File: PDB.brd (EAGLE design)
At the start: 126.8 x 162.5 mm, 49 parts, among them J1 B06B-HCMKK, J2 B06B-HCMKK, J3 SS-6488-NF-A431, J4 SS-6488-NF-A431, J5 B06B-HCMKK, J6 B03B-HCMKS, J7 B03B-HCMKS, J8 SS-6488-NF-A431

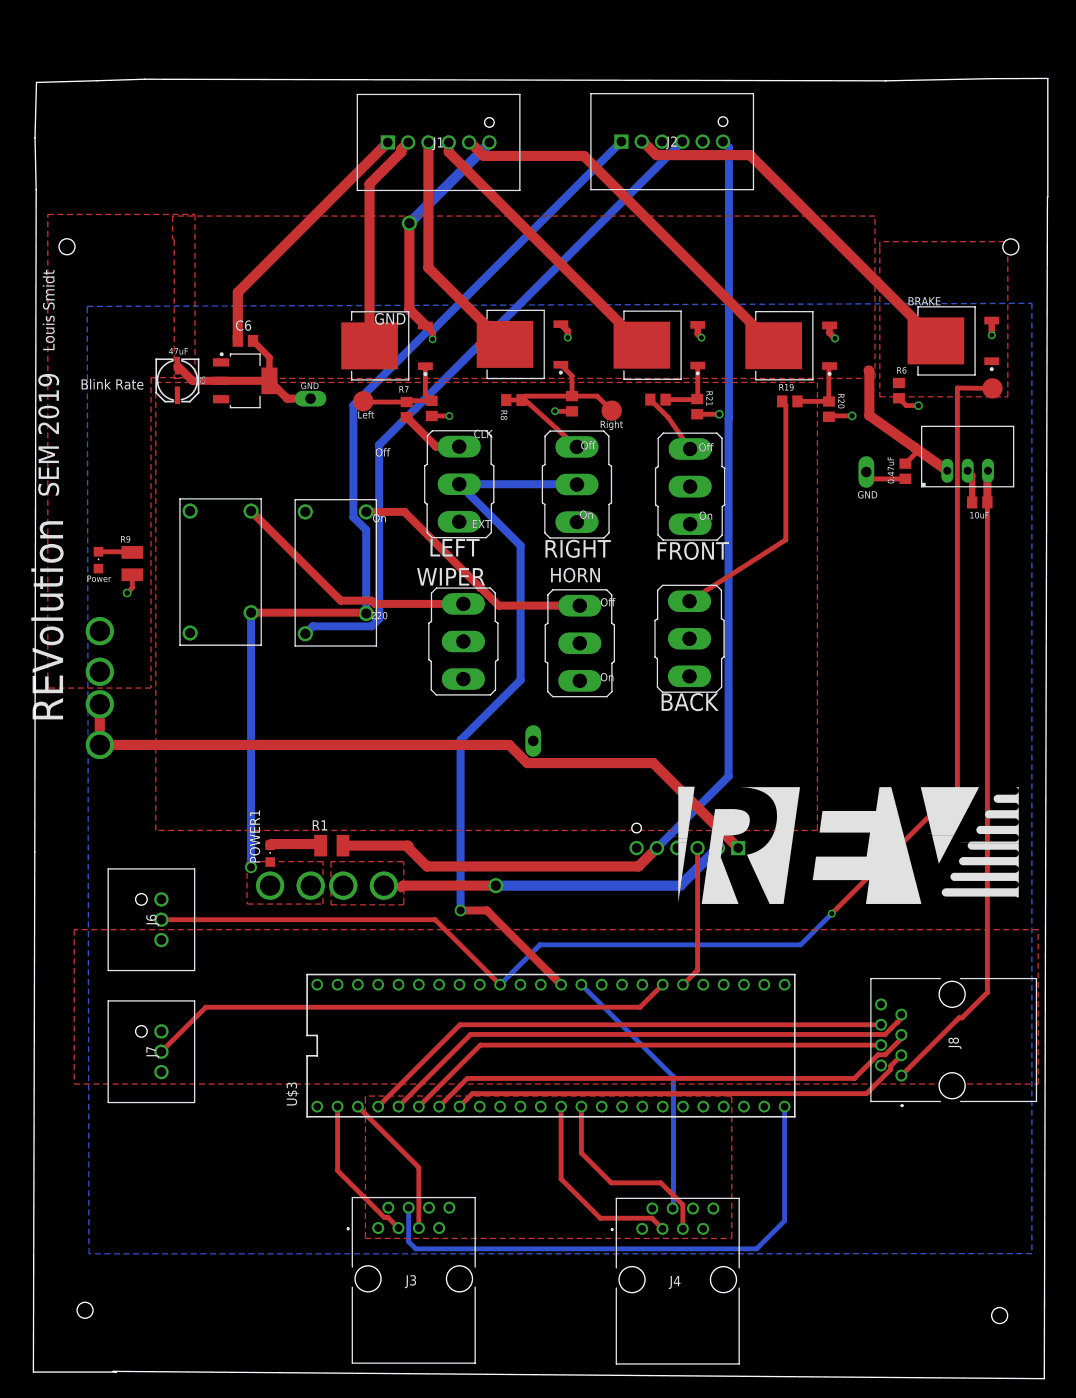
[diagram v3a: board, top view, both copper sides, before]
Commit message: Decorative modification
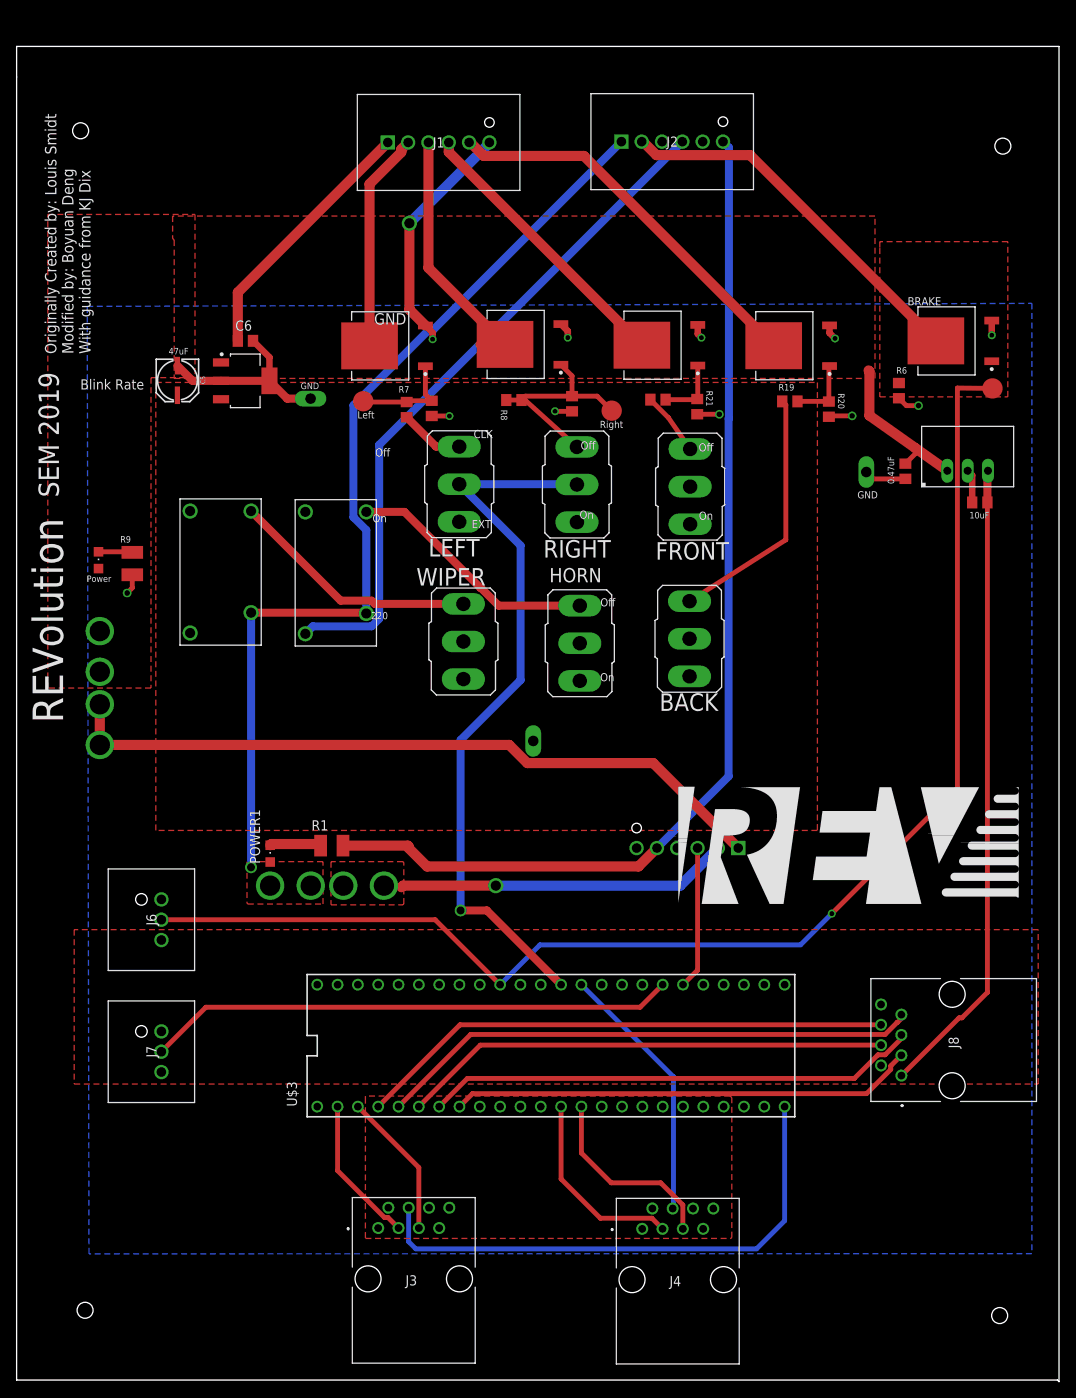
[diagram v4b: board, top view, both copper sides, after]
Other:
- board size 126.8 x 162.5 mm -> 130.3 x 166.9 mm
- board text added: "Originally Created by: Louis Smidt Modified by: Boyuan Deng With guidance from KJ Dix"
- board text removed: "Louis Smidt"
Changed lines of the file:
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@@
 <board>
 <plain>
-<wire x1="130.3613875" y1="-11.928015625" x2="130.75645" y2="135.749278125" width="0" layer="20"/>
-<wire x1="130.75645" y1="135.749278125" x2="130.8" y2="135.792828125" width="0" layer="20"/>
-<wire x1="130.8" y1="135.792828125" x2="130.8" y2="150.6" width="0" layer="20"/>
-<wire x1="130.8" y1="150.6" x2="123.665928125" y2="150.570725" width="0" layer="20"/>
-<wire x1="123.665928125" y1="150.570725" x2="110.536653125" y2="150.3" width="0" layer="20"/>
-<wire x1="110.536653125" y1="150.3" x2="17.9" y2="150.5" width="0" layer="20"/>
-<wire x1="17.9" y1="150.5" x2="12" y2="150.31475" width="0" layer="20"/>
-<wire x1="12" y1="150.31475" x2="4.38525" y2="150.1" width="0" layer="20"/>
-<wire x1="4.38525" y1="150.1" x2="4.2" y2="143.2" width="0" layer="20"/>
-<wire x1="4.2" y1="143.2" x2="4.346496875" y2="136.691890625" width="0" layer="20"/>
-<wire x1="4.346496875" y1="136.691890625" x2="4.1724375" y2="53.904" width="0" layer="20"/>
-<wire x1="4.1724375" y1="53.904" x2="4" y2="-11.1" width="0" layer="20"/>
-<wire x1="4" y1="-11.1" x2="14.380440625" y2="-11.1" width="0" layer="20"/>
-<wire x1="14.380440625" y1="-11.1" x2="13.96286875" y2="-11.017571875" width="0" layer="20"/>
-<wire x1="13.96286875" y1="-11.017571875" x2="130.3613875" y2="-11.928015625" width="0" layer="20"/>
 <text x="37.404" y="111.766" size="0.8128" layer="25">GND</text>
 <text x="9.862" y="111.718" size="1.27" layer="25">Blink Rate</text>
@@
 <rectangle x1="114.93" y1="61.99" x2="122.21" y2="62.01" layer="25"/>
 <rectangle x1="126.79" y1="61.99" x2="127.17" y2="62.01" layer="25"/>
-<hole x="8.2" y="129.56" drill="2"/>
+<hole x="9.9" y="144.06" drill="2"/>
 <hole x="10.46" y="-3.38" drill="2"/>
-<hole x="126.18" y="129.54" drill="2"/>
+<hole x="125.18" y="142.14" drill="2"/>
 <hole x="124.78" y="-4.04" drill="2"/>
-<text x="6.64" y="116.46" size="1.4224" layer="25" rot="R90">Louis Smidt</text>
+<text x="11.14" y="116.16" size="1.4224" layer="25" rot="R90">Originally Created by: Louis Smidt
+Modified by: Boyuan Deng
+With guidance from KJ Dix</text>
 <text x="10.66" y="87.66" size="0.8128" layer="25">Power</text>
 <text x="61.42" y="106.66" size="1.016" layer="25" rot="R180">CLK</text>
@@
 <text x="20.9" y="116.1" size="0.8128" layer="25">47uF</text>
 <text x="111.6" y="99.9" size="0.8128" layer="25" rot="R90">0.47uF</text>
+<wire x1="1.9" y1="150.8" x2="1.9" y2="150.7" width="0.1524" layer="20"/>
+<wire x1="1.9" y1="150.7" x2="1.9" y2="-12.1" width="0.1524" layer="20"/>
+<wire x1="1.9" y1="-12.1" x2="132" y2="-12.1" width="0.1524" layer="20"/>
+<wire x1="132" y1="-12.1" x2="132.2" y2="-12.3" width="0.1524" layer="20"/>
+<wire x1="132.2" y1="-12.3" x2="132.2" y2="154.6" width="0.1524" layer="20"/>
+<wire x1="132.2" y1="154.6" x2="1.9" y2="154.6" width="0.1524" layer="20"/>
+<wire x1="1.9" y1="154.6" x2="1.9" y2="150.8" width="0.1524" layer="20"/>
 </plain>
 <attributes>
@@
 <vertex x="109.8" y="110.8"/>
 <vertex x="125.8" y="110.8"/>
-<vertex x="125.8" y="129.4"/>
-<vertex x="126.6" y="130.2"/>
+<vertex x="125.8" y="130.2"/>
 <vertex x="109.8" y="130.2"/>
 </polygon>
@@
 </drawing>
 <compatibility>
+<note version="6.3" minversion="6.2.2" severity="warning">
+Since Version 6.2.2 text objects can contain more than one line,
+which will not be processed correctly with this version.
+</note>
 <note version="8.2" severity="warning">
 Since Version 8.2, EAGLE supports online libraries. The ids

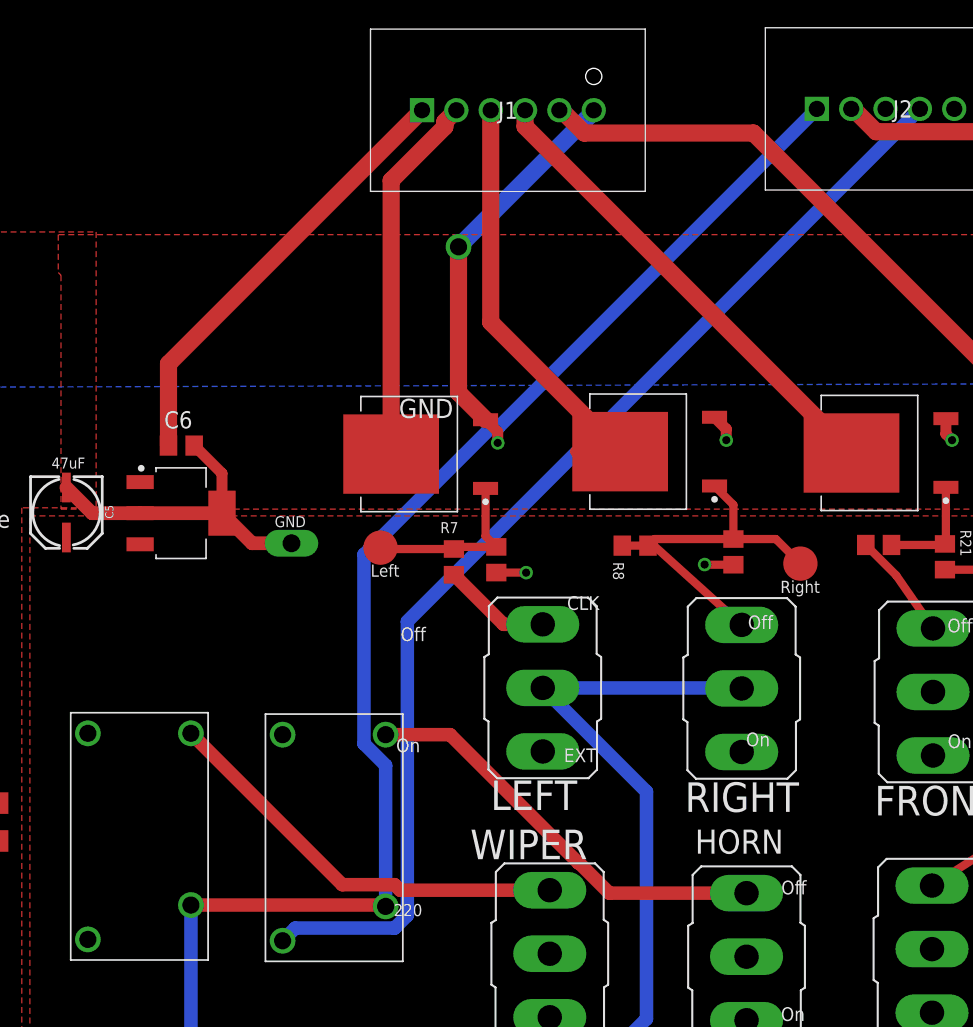
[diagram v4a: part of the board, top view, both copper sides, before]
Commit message: VIPER misspelling corrected
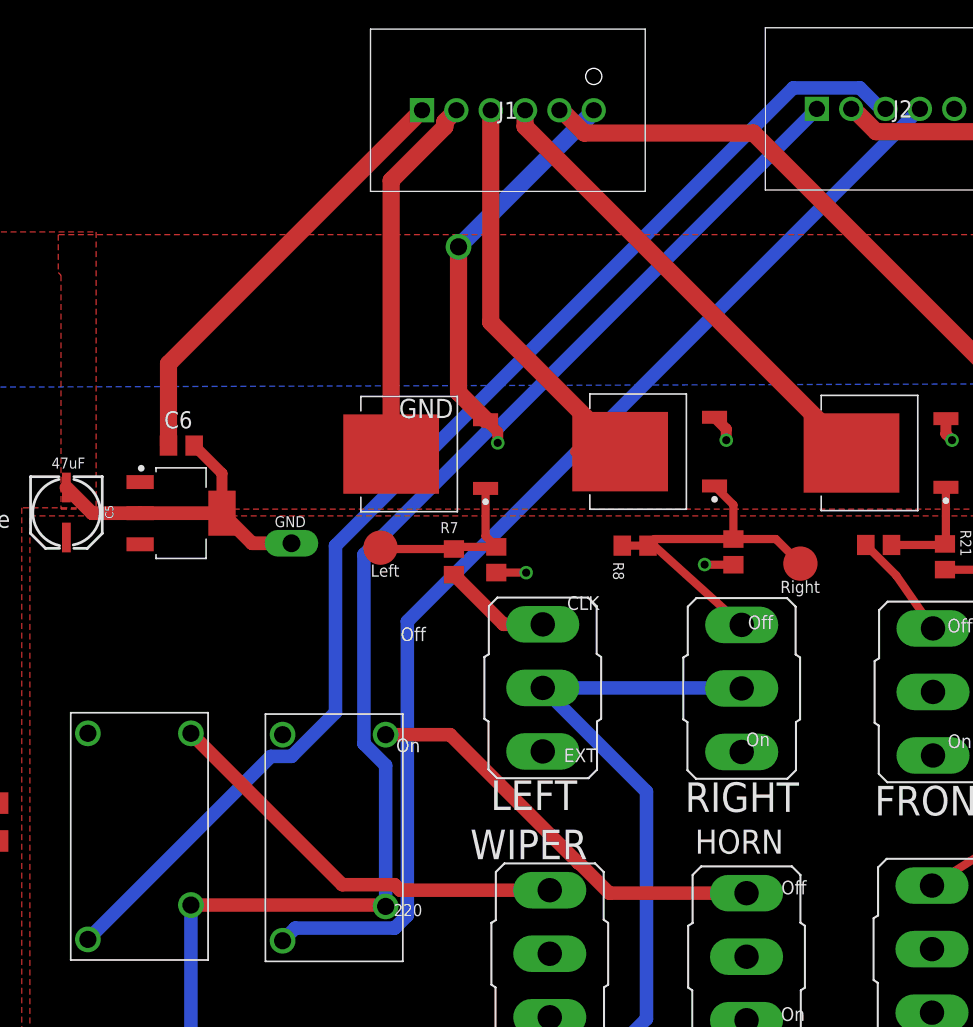
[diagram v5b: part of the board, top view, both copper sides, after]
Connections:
- removed net VIPER: J2.3
- net WIPER: now also J2.3
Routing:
- net WIPER: track 0.00 -> 92.9 mm
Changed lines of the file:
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@@
 <signal name="WIPER">
 <contactref element="U$6" pad="SWB"/>
+<contactref element="J2" pad="3"/>
+<wire x1="23.59" y1="81.28" x2="37.1251" y2="94.8151" width="1" layer="16"/>
+<wire x1="37.1251" y1="94.8151" x2="38.654775" y2="94.8151" width="1" layer="16"/>
+<wire x1="38.654775" y1="94.8151" x2="41.9" y2="98.060325" width="1" layer="16"/>
+<wire x1="41.9" y1="98.060325" x2="41.9" y2="110.4" width="1" layer="16"/>
+<wire x1="82.23543125" y1="142.7" x2="82.58" y2="142.7" width="1" layer="16"/>
+<wire x1="80.68303125" y1="144.2524" x2="82.23543125" y2="142.7" width="1" layer="16"/>
+<wire x1="41.9" y1="110.4" x2="75.7524" y2="144.2524" width="1" layer="16"/>
+<wire x1="75.7524" y1="144.2524" x2="80.68303125" y2="144.2524" width="1" layer="16"/>
 </signal>
 <signal name="HORN">
@@
 <wire x1="58.88" y1="23.7" x2="108.14160625" y2="23.7" width="0.6096" layer="1"/>
 </signal>
-<signal name="VIPER">
-<contactref element="J2" pad="3"/>
-</signal>
 </signals>
